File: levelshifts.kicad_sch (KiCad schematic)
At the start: 18 parts, among them U12 SSM6N7002KFU, U14 SSM6N7002KFU, U15 SSM6N7002KFU, U16 SSM6N7002KFU

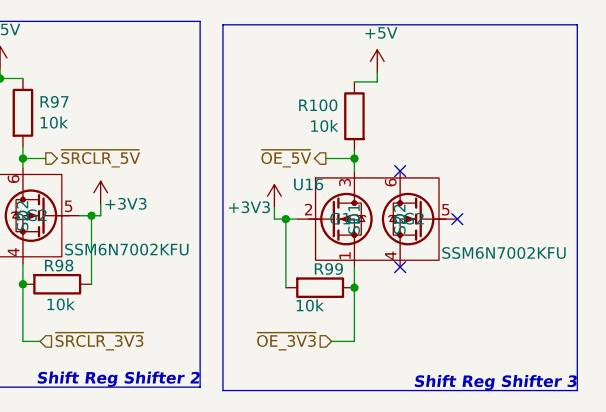
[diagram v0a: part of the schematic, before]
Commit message: More schematic updates
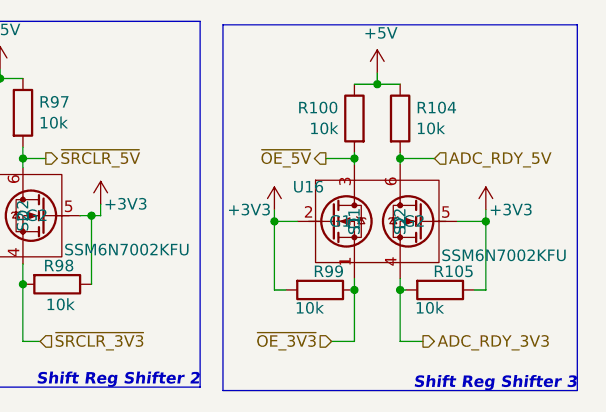
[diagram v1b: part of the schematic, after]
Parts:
- added R104, R105: 10k, Resistor_SMD:R_0402_1005Metric, symbol Device:R
- R100, R21, R23, R24, R9, R91, R92, R93, R94, R95, R96, R97, R98, R99: footprint Resistor_SMD:R_0603_1608Metric_Pad0.98x0.95mm_HandSolder -> Resistor_SMD:R_0402_1005Metric
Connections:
- net +3V3: now also U16.5 (G2), R105.1
- net +5V: now also R104.1
- net ADC_RDY_3V3: now reaches U16.4 (S2)
- net ADC_RDY_3V3: now also R105.2
- net ADC_RDY_5V: now reaches U16.6 (D2)
- net ADC_RDY_5V: now also R104.2
- no-connect marks 3 -> 0

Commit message: Updated all of component values
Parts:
- R100, R104, R105, R91, R92, R93, R94, R95, R96, R97, R98, R99: Comment (none) -> 10 kOhms ±1% 0.063W, 1/16W Chip Resistor 0402 (1005 Metric)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; Digikey Number (none) -> 311-10.0KLRCT-ND; Part Number (none) -> RC0402FR-0710KL; Price ($) (none) -> 0.1
- R21, R23, R24, R9: Comment (none) -> 2.2 kOhms ±1% 0.063W, 1/16W Chip Resistor 0402 (1005 Metric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; Digikey Number (none) -> 311-2.20KLRCT-ND; Part Number (none) -> RC0402FR-072K2L; Price ($) (none) -> 0.1

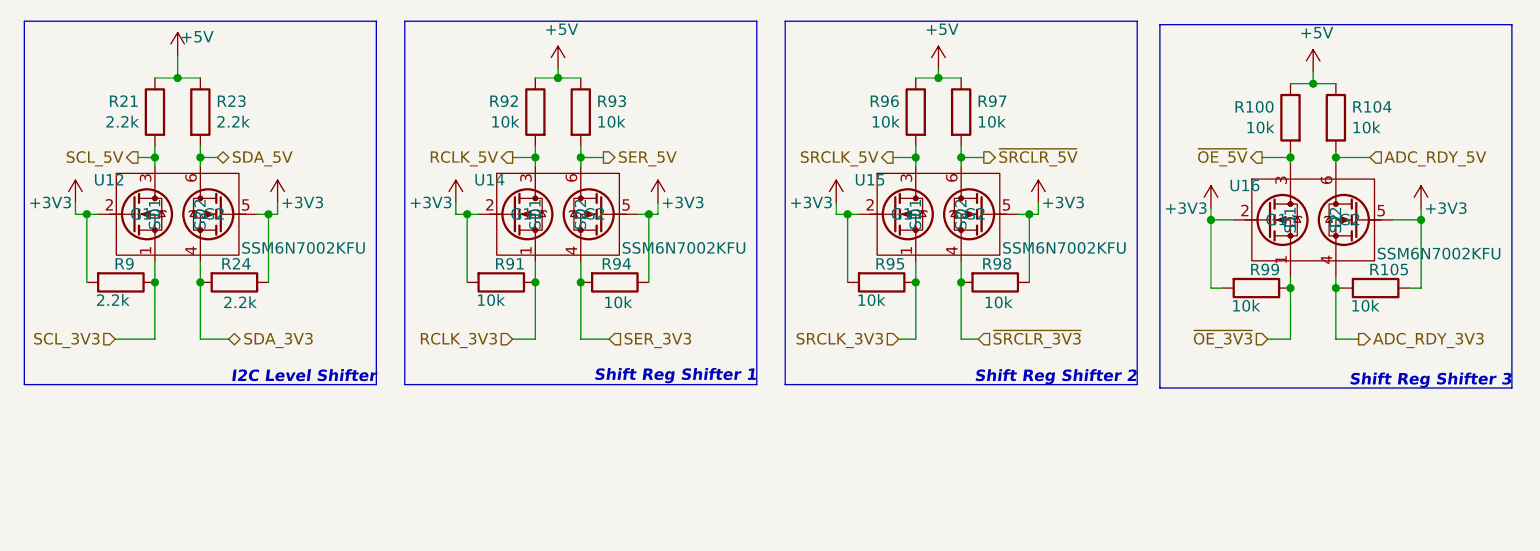
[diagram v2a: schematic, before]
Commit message: ALMOST THERE
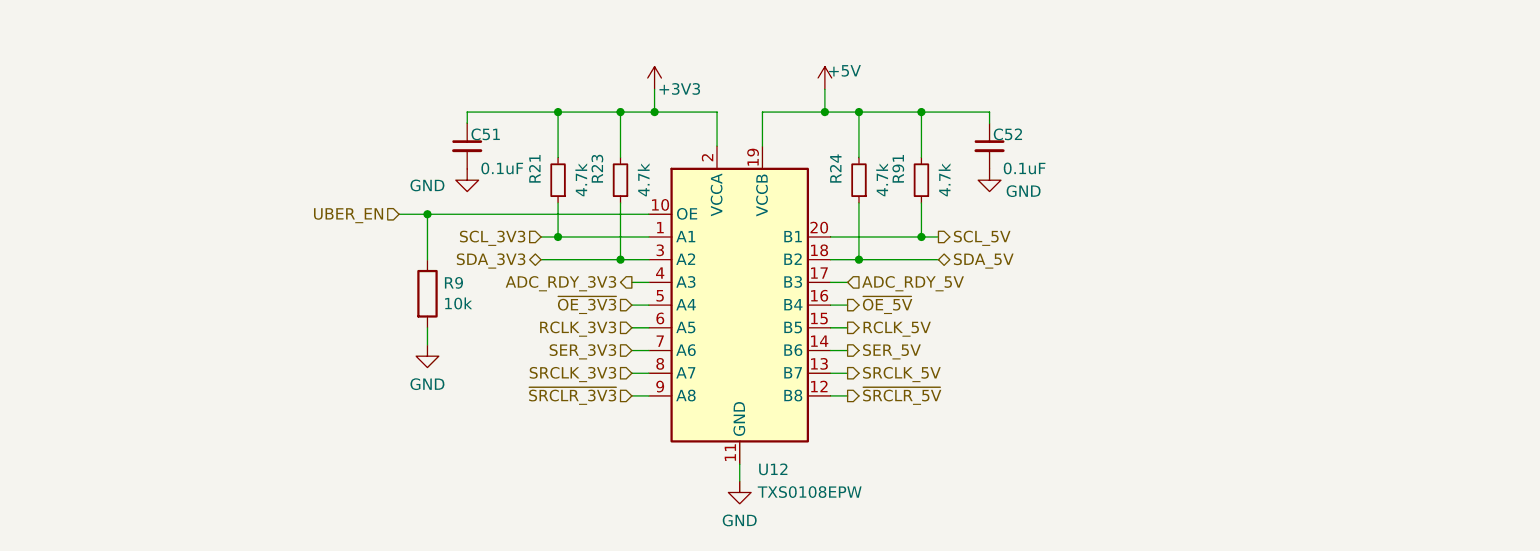
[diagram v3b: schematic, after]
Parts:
- removed R100, R104, R105, R91, R92, R93, R94, R95, R96, R97, R98, R99: 10k, Resistor_SMD:R_0402_1005Metric, symbol Device:R
- removed R21, R23, R24: 2.2k, Resistor_SMD:R_0402_1005Metric, symbol Device:R
- removed U12, U14, U15, U16: SSM6N7002KFU, Package_TO_SOT_SMD:SOT-363_SC-70-6, symbol ClementsSymbols:SSM6N7002KFU
- added C51, C52: 0.1uF, Capacitor_SMD:C_0402_1005Metric, symbol Device:C_Small
- added R21, R23, R24, R91: 4.7k, Resistor_SMD:R_0402_1005Metric, symbol Device:R_Small
- added U12: TXS0108EPW, Package_SO:TSSOP-20_4.4x6.5mm_P0.65mm, symbol Logic_LevelTranslator:TXS0108EPW
- R9: value 2.2k -> 10k; Comment 2.2 kOhms ±1% 0.063W, 1/16W Chip Resistor 0402 (1005 Metric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 -> 10 kOhms ±1% 0.063W, 1/16W Chip Resistor 0402 (1005 Metric)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; Digikey Number 311-2.20KLRCT-ND -> 311-10.0KLRCT-ND; Part Number RC0402FR-072K2L -> RC0402FR-0710KL
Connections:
- net +3V3: now also C51.1, R21.2, R23.2, U12.2 (VCCA); no longer R9.2
- net +5V: now also C52.1, R24.2, R91.2, U12.19 (VCCB)
- net ADC_RDY_3V3: now also U12.4 (A3)
- net ADC_RDY_5V: now also U12.17 (B3)
- net RCLK_3V3: now also U12.6 (A5)
- net RCLK_5V: now also U12.15 (B5)
- net SCL_3V3: now also R21.1, U12.1 (A1); no longer R9.1
- net SCL_5V: now also R91.1, U12.20 (B1)
- net SDA_3V3: now also R23.1, U12.3 (A2)
- net SDA_5V: now also R24.1, U12.18 (B2)
- net SER_3V3: now also U12.7 (A6)
- net SER_5V: now also U12.14 (B6)
- net SRCLK_3V3: now also U12.8 (A7)
- net SRCLK_5V: now also U12.13 (B7)
- net ~{OE_3V3}: now also U12.5 (A4)
- net ~{OE_5V}: now also U12.16 (B4)
- net ~{SRCLR_3V3}: now also U12.9 (A8)
- net ~{SRCLR_5V}: now also U12.12 (B8)
- new net GND: C51.2, C52.2, R9.2, U12.11 (GND)
- new net UBER_EN: R9.1, U12.10 (OE)
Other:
- note removed: "I2C Level Shifter"
- note removed: "Shift Reg Shifter 1"
- note removed: "Shift Reg Shifter 2"
- note removed: "Shift Reg Shifter 3"
